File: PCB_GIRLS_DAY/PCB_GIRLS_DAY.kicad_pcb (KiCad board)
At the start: 2 copper layers, 72.1 x 66.5 mm, 84 parts, among them J1 USB_B_Micro, J2 Conn_01x04_Pin, J3 Conn_01x03_Pin, J4 Conn_01x03_Pin, J5 Conn_02x20_Odd_Even, Q1 S8050, Q2 2SC3357-T1-A, Q3 MMBT918, SW1 SW_SPDT, U1 STM32F446RETx, U3 AP2112K-3.3, U4 AMS1117-5.0, U5 SB7343392TT, U6 LM358_C5252902, X1 X50328MSB2GI

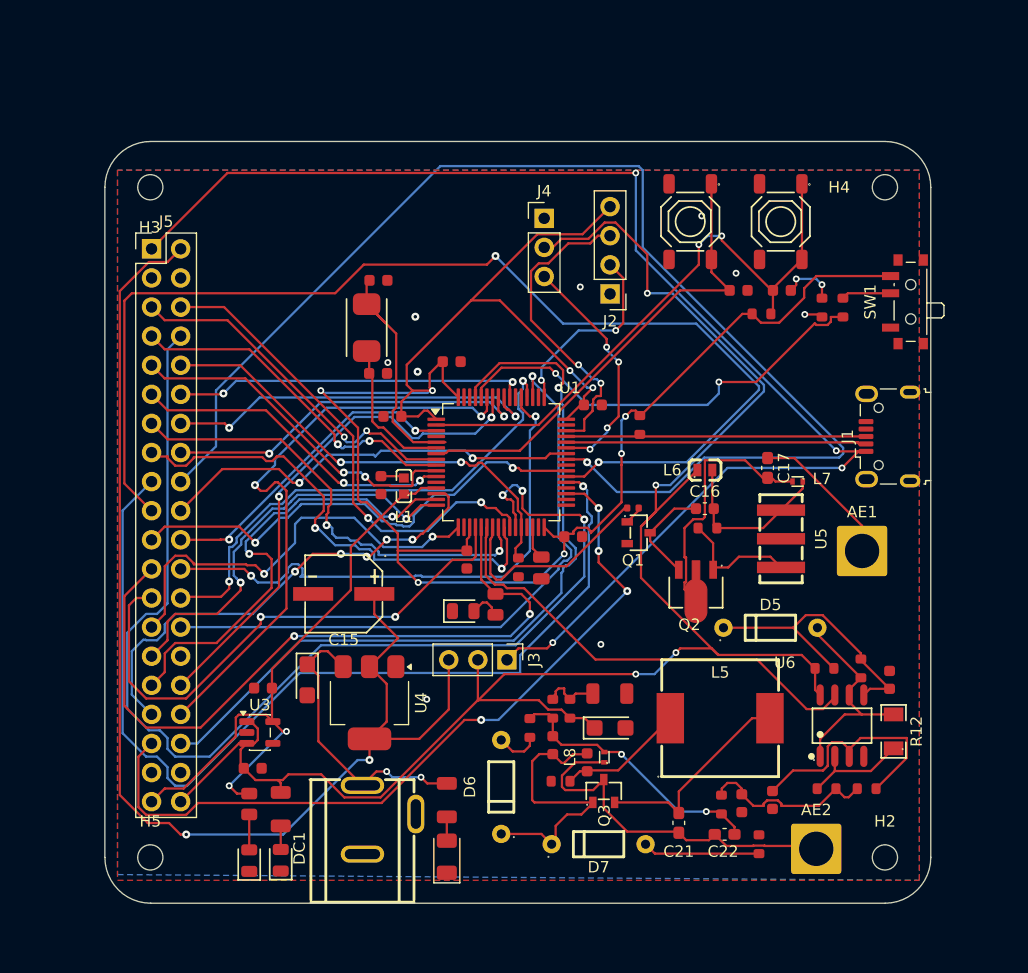
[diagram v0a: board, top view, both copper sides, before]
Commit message: PCB revision Cyprien
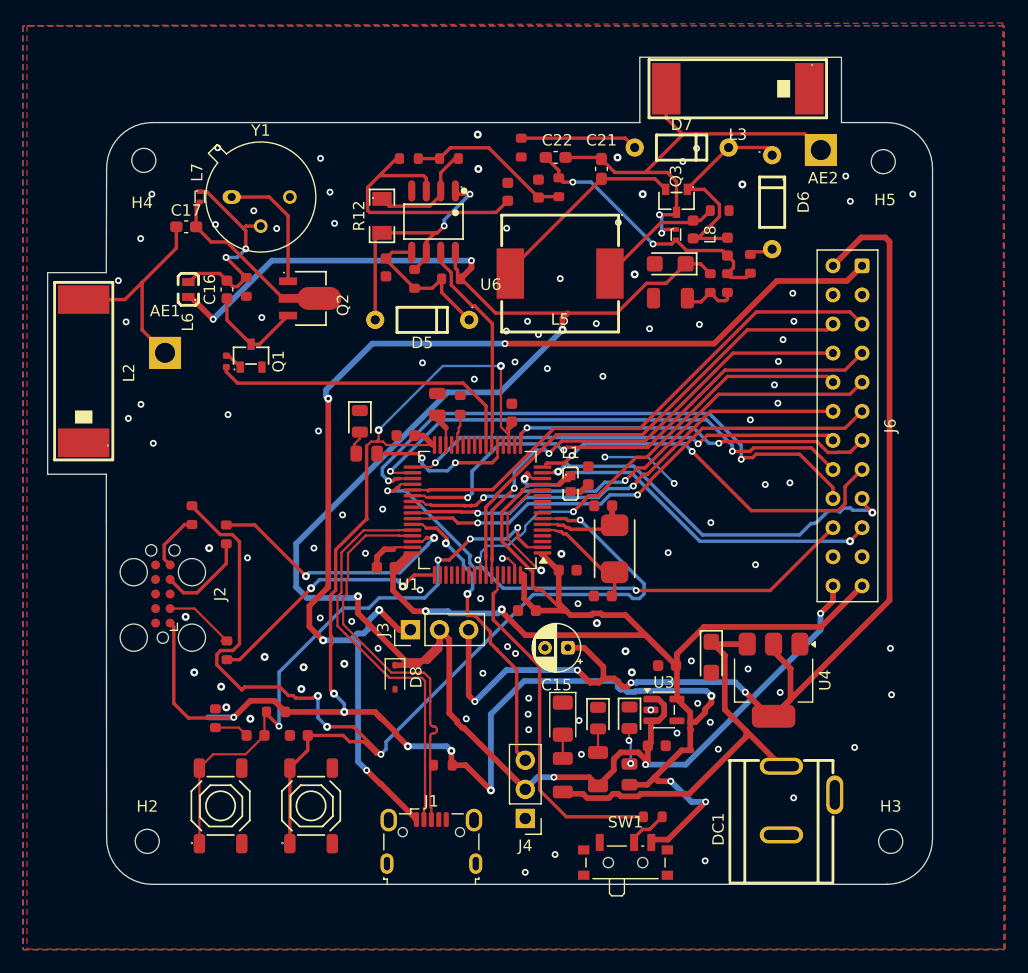
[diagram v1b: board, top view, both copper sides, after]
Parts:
- removed J5: Conn_02x20_Odd_Even, Connector_PinHeader_2.54mm:PinHeader_2x20_P2.54mm_Vertical
- removed U5: SB7343392TT, EasyEDA:CRYSTAL-SMD_3P-L7.7-W3.7-P2.50_SB7343392TT
- added D8: D_Schottky, Diode_SMD:D_SOD-323, F.Cu at (125.2, 109.3)
- added J6: Conn_02x12_Odd_Even, Connector_Samtec_HLE_THT:Samtec_HLE-112-02-xx-DV-TE_2x12_P2.54mm_Horizontal, F.Cu at (166.0, 73.4)
- added L2: BW433MNX1304, EasyEDA:ANT-SMD_L130-W42_BW433MNX, F.Cu at (98.0, 82.5)
- added L3: BW433MNX1304, EasyEDA:ANT-SMD_L130-W42_BW433MNX, F.Cu at (155.2, 57.9)
- added R23: 22Ω, PCM_JLCPCB:R_0603, F.Cu at (110.5, 106.9)
- added R25: 22Ω, PCM_JLCPCB:R_0603, F.Cu at (110.5, 96.8)
- added R26: 22Ω, PCM_JLCPCB:R_0603, F.Cu at (107.5, 95.1)
- added Y1: Crystal_GND3, Package_TO_SOT_THT:TO-39-3, F.Cu at (111.0, 67.3)
- AE1, AE2: footprint Connector_Wire:SolderWire-2.5sqmm_1x01_D2.4mm_OD4.4mm -> Connector_Samtec_HPM_THT:Samtec_HPM-01-01-x-S_Straight_1x01_Pitch5.08mm
- C15: footprint EasyEDA-CAP_22uF_Aluminium:CAP-SMD_BD6.3-L6.6-W6.6-FD -> Capacitor_THT:CP_Radial_D4.0mm_P2.00mm
- H2, H3, H4, H5: footprint MountingHole:MountingHole_2.2mm_M2 -> MountingHole:MountingHole_2.1mm
- J2: value Conn_01x04_Pin -> Conn_02x05_Counter_Clockwise; footprint Connector_PinHeader_2.54mm:PinHeader_1x04_P2.54mm_Vertical -> Connector:Tag-Connect_TC2050-IDC-FP_2x05_P1.27mm_Vertical
- moved H5 88.2 mm to (167.8, 64.3)
- moved H3 86.3 mm to (168.5, 123.6)
- moved S1 70.7 mm to (110.0, 120.5), turned to 90 degrees
- moved R14 68.0 mm to (126.4, 64.0), turned to 180 degrees
- moved H4 64.7 mm to (103.3, 64.2)
- moved H2 64.4 mm to (103.6, 123.6)
- moved R19 64.3 mm to (136.2, 63.0), turned to -90 degrees
- moved R13 64.1 mm to (129.9, 64.0), turned to 0 degrees
- moved R5 63.9 mm to (109.5, 112.8), turned to -90 degrees
- moved R12 63.4 mm to (124.1, 69.0), turned to -90 degrees
- moved AE1 63.3 mm to (105.2, 81.0)
- moved D7 61.2 mm to (150.2, 63.0), turned to 180 degrees
- moved AE2 61.0 mm to (162.4, 63.2)
- moved C22 60.9 mm to (139.2, 63.9), turned to 180 degrees
- moved S2 60.8 mm to (117.9, 120.5), turned to 90 degrees
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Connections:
- net /SCH_MCU/PB2 renamed Net-(U1-PB2)
- net /SCH_MCU/USB_D- renamed /SCH_MCU/USB_DN
- J1 pad 3: /SCH_MCU/USB_D+ -> /SCH_MCU/USB_DP
- J1 pad SH: unconnected-(J1-Shield-PadSH) -> GND
- J2 pad 1: GND -> +3V3
- J2 pad 2: /SCH_MCU/SWCLK -> Net-(J2-Pin_2)
- J2 pad 3: /SCH_MCU/SWDIO -> GND
- J2 pad 4: +3V3 -> Net-(J2-Pin_4)
- R22 pad 1: /SCH_MCU/USB_D+ -> +3V3
- R22 pad 2: +3V3 -> /SCH_MCU/USB_DP
- U1 pad 10: /SCH_MCU/PC2 -> unconnected-(U1-PC2-Pad10)
- U1 pad 11: /SCH_MCU/PC3 -> unconnected-(U1-PC3-Pad11)
- U1 pad 20: /SCH_MCU/PA4 -> unconnected-(U1-PA4-Pad20)
- U1 pad 24: /SCH_MCU/PC4 -> unconnected-(U1-PC4-Pad24)
- U1 pad 25: /SCH_MCU/PC5 -> unconnected-(U1-PC5-Pad25)
- U1 pad 26: /SCH_MCU/PB0 -> unconnected-(U1-PB0-Pad26)
- U1 pad 27: /SCH_MCU/PB1 -> unconnected-(U1-PB1-Pad27)
- U1 pad 3: /SCH_MCU/PC14 -> unconnected-(U1-PC14-Pad3)
- U1 pad 33: unconnected-(U1-PB12-Pad33) -> /SCH_MCU/PB12
- U1 pad 34: unconnected-(U1-PB13-Pad34) -> /SCH_MCU/PB13
- U1 pad 36: unconnected-(U1-PB15-Pad36) -> /SCH_MCU/PB15
- U1 pad 45: /SCH_MCU/USB_D+ -> /SCH_MCU/USB_DP
- U1 pad 51: /SCH_MCU/PC10 -> unconnected-(U1-PC10-Pad51)
- U1 pad 52: /SCH_MCU/PC11 -> unconnected-(U1-PC11-Pad52)
- U1 pad 53: /SCH_MCU/PC12 -> unconnected-(U1-PC12-Pad53)
- U1 pad 55: /SCH_MCU/PB3 -> unconnected-(U1-PB3-Pad55)
- U1 pad 56: /SCH_MCU/PB4 -> unconnected-(U1-PB4-Pad56)
- U1 pad 61: /SCH_MCU/PB8 -> unconnected-(U1-PB8-Pad61)
- U1 pad 8: /SCH_MCU/PC0 -> unconnected-(U1-PC0-Pad8)
- U1 pad 9: /SCH_MCU/PC1 -> unconnected-(U1-PC1-Pad9)
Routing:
- net /SCH_MCU/PB1: track 101.8 -> 0.00 mm, vias 3 -> 0
- net /SCH_MCU/PA8: track 113.5 -> 40.6 mm, vias 1 -> 2
- net /SCH_MCU/PB8: track 69.2 -> 0.00 mm, vias 1 -> 0
- net /SCH_MCU/PC10: track 55.8 -> 0.00 mm, vias 1 -> 0
- net /SCH_MCU/PC7: track 101.3 -> 46.1 mm
- net /SCH_MCU/NRST: track 41.5 -> 95.6 mm, vias 0 -> 4
- net /SCH_MCU/LED: track 64.0 -> 13.0 mm
- net /SCH_MCU/PC12: track 48.4 -> 0.00 mm, vias 2 -> 0
- net /SCH_MCU/PA4: track 47.8 -> 0.00 mm, vias 2 -> 0
- net /SCH_MCU/PB15: track 0.00 -> 47.8 mm, vias 0 -> 2
- net /SCH_MCU/PB13: track 0.00 -> 44.8 mm, vias 0 -> 2
- net /SCH_MCU/PC11: track 44.0 -> 0.00 mm, vias 2 -> 0
- net /SCH_MCU/PB0: track 43.6 -> 0.00 mm, vias 2 -> 0
- net /SCH_MCU/PC5: track 42.7 -> 0.00 mm, vias 2 -> 0
- net /SCH_MCU/PC4: track 40.4 -> 0.00 mm, vias 2 -> 0
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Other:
- board size 72.1 x 66.5 mm -> 77.2 x 72.2 mm
